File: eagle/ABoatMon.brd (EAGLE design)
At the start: 57.5 x 36.2 mm, 17 parts, among them J1 5V, J2 GND, J3 GND

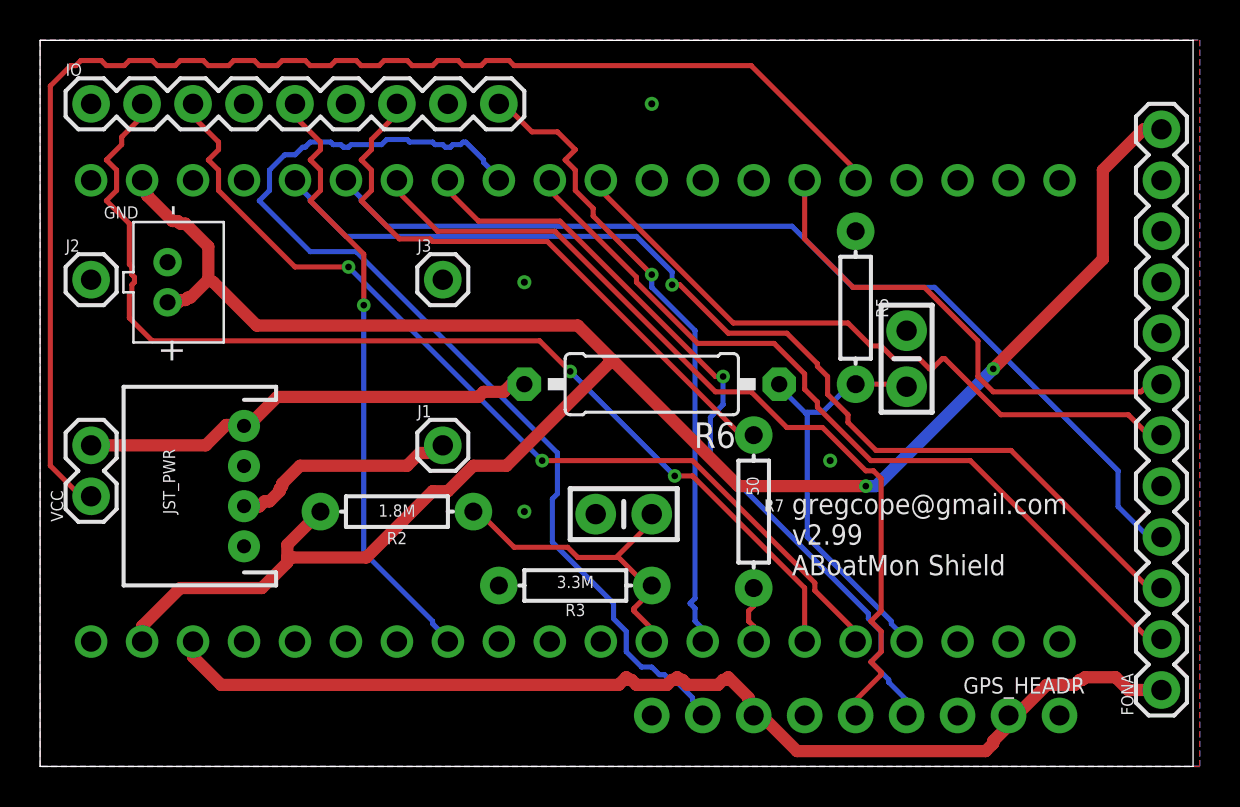
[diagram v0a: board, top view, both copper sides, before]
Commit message: doco added
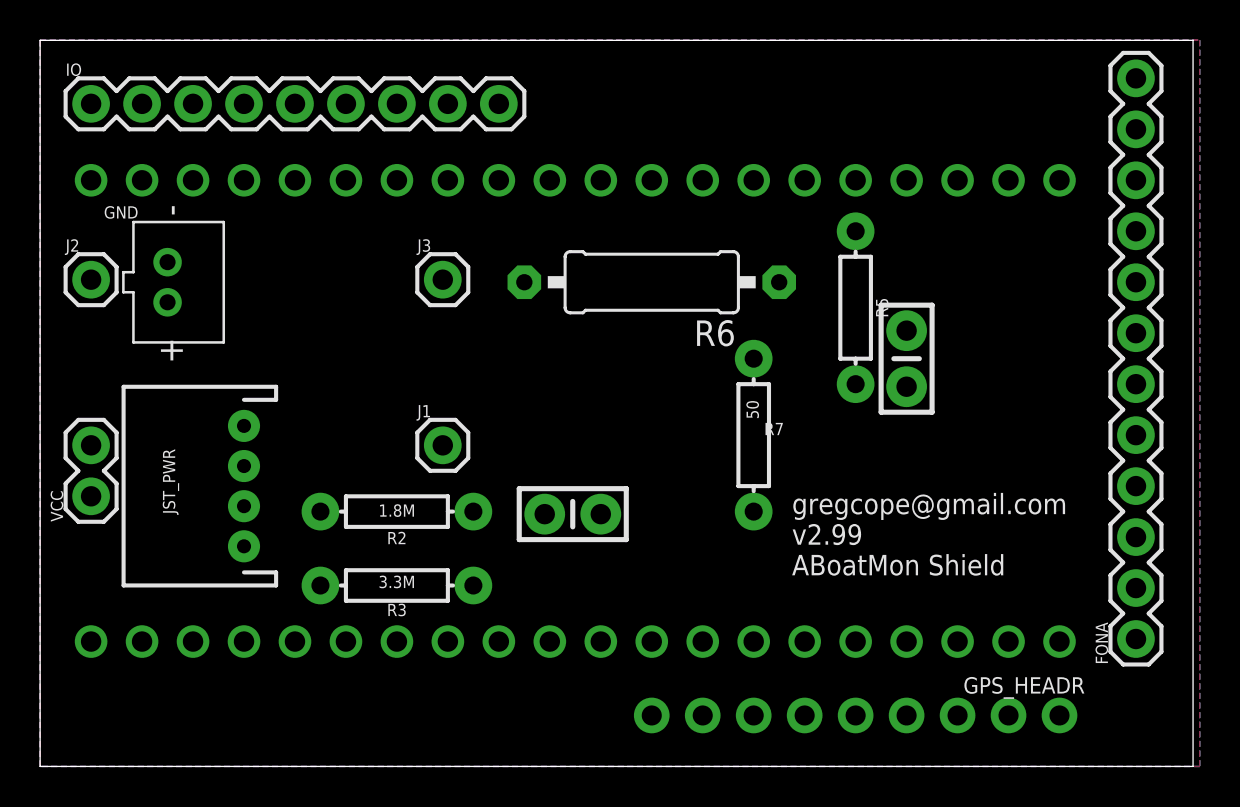
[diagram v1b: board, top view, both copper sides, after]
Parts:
- moved R3 8.89 mm to (17.8, 9.02)
- moved R6 5.08 mm to (30.5, 24.1)
- moved R7 3.81 mm to (35.6, 16.5)
- moved FONA 2.84 mm to (54.6, 6.35)
- moved C1 2.54 mm to (26.5, 12.6)
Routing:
- net VIN: track 103.7 -> 0.00 mm, vias 2 -> 0
- net D19_PWRON: track 66.7 -> 0.00 mm
- net 3.3V: track 54.5 -> 0.00 mm
- net D27_DS_PWR: track 54.4 -> 0.00 mm, vias 2 -> 0
- net D8_FONA_TX: track 52.9 -> 0.00 mm, vias 1 -> 0
- net D12_GPS_ENABLE: track 52.2 -> 0.00 mm
- net D9_FONA_RX: track 49.2 -> 0.00 mm
- net D28_DS_DATA: track 46.8 -> 0.00 mm, vias 2 -> 0
- net D10_GPS_RX: track 43.8 -> 0.00 mm
- net D13_FONA_NETSTAT: track 41.0 -> 0.00 mm
- net D11_GPS_TX: track 39.7 -> 0.00 mm, vias 1 -> 0
- net D14_FONA_KEY: track 33.9 -> 0.00 mm
- net D25_LED_SWITCH: track 32.5 -> 0.00 mm, vias 1 -> 0
- net D3_BILGESW: track 30.8 -> 0.00 mm, vias 1 -> 0
- net N$2: track 30.4 -> 0.00 mm
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
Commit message: rollback
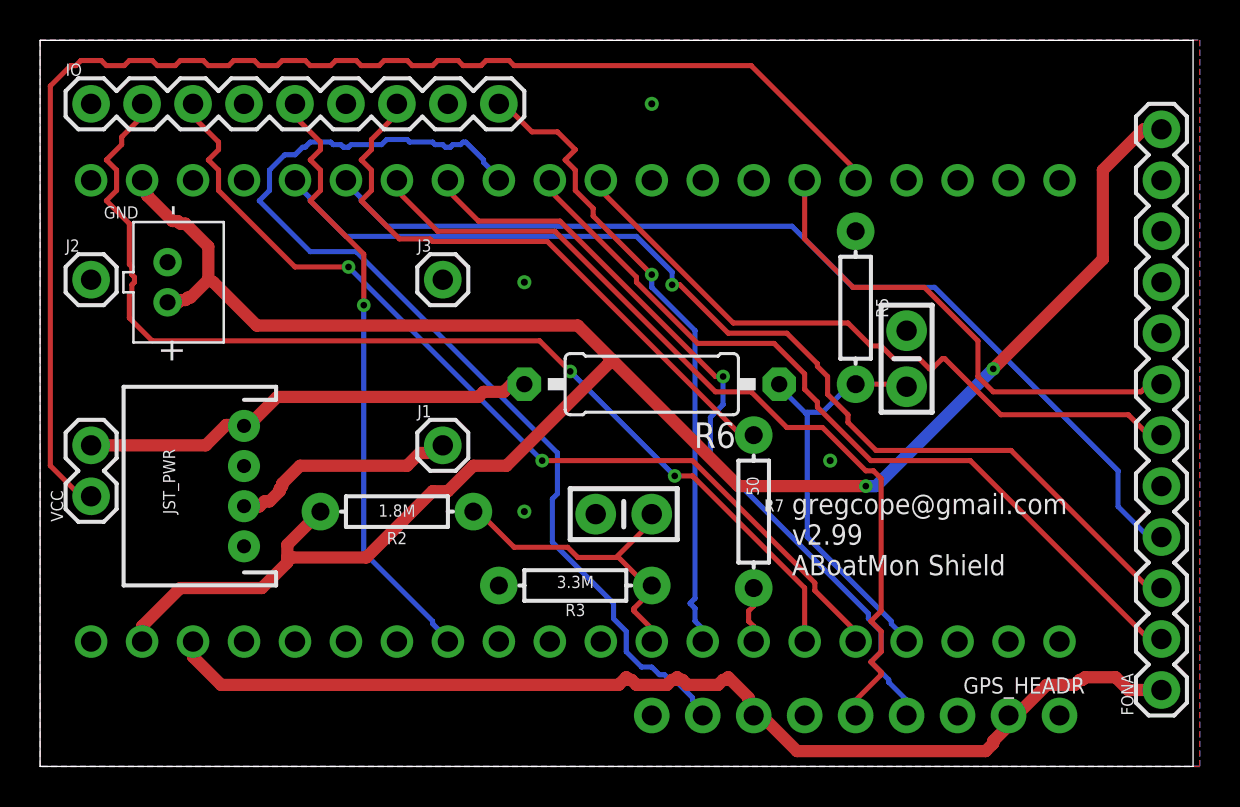
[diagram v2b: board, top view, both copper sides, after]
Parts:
- moved R3 8.89 mm to (26.7, 9.02)
- moved R6 5.08 mm to (30.5, 19.1)
- moved R7 3.81 mm to (35.6, 12.7)
- moved FONA 2.84 mm to (55.9, 3.81)
- moved C1 2.54 mm to (29.1, 12.6)
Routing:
- net VIN: track 0.00 -> 103.7 mm, vias 0 -> 2
- net D19_PWRON: track 0.00 -> 66.7 mm
- net 3.3V: track 0.00 -> 54.5 mm
- net D27_DS_PWR: track 0.00 -> 54.4 mm, vias 0 -> 2
- net D8_FONA_TX: track 0.00 -> 52.9 mm, vias 0 -> 1
- net D12_GPS_ENABLE: track 0.00 -> 52.2 mm
- net D9_FONA_RX: track 0.00 -> 49.2 mm
- net D28_DS_DATA: track 0.00 -> 46.8 mm, vias 0 -> 2
- net D10_GPS_RX: track 0.00 -> 43.8 mm
- net D13_FONA_NETSTAT: track 0.00 -> 41.0 mm
- net D11_GPS_TX: track 0.00 -> 39.7 mm, vias 0 -> 1
- net D14_FONA_KEY: track 0.00 -> 33.9 mm
- net D25_LED_SWITCH: track 0.00 -> 32.5 mm, vias 0 -> 1
- net D3_BILGESW: track 0.00 -> 30.8 mm, vias 0 -> 1
- net N$2: track 0.00 -> 30.4 mm
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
